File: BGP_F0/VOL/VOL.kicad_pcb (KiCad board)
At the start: 2 copper layers, 20 x 26 mm, 4 parts, among them J1 Conn_01x03_Female, J2 Conn_01x03_Female, P1 CONN_01X02

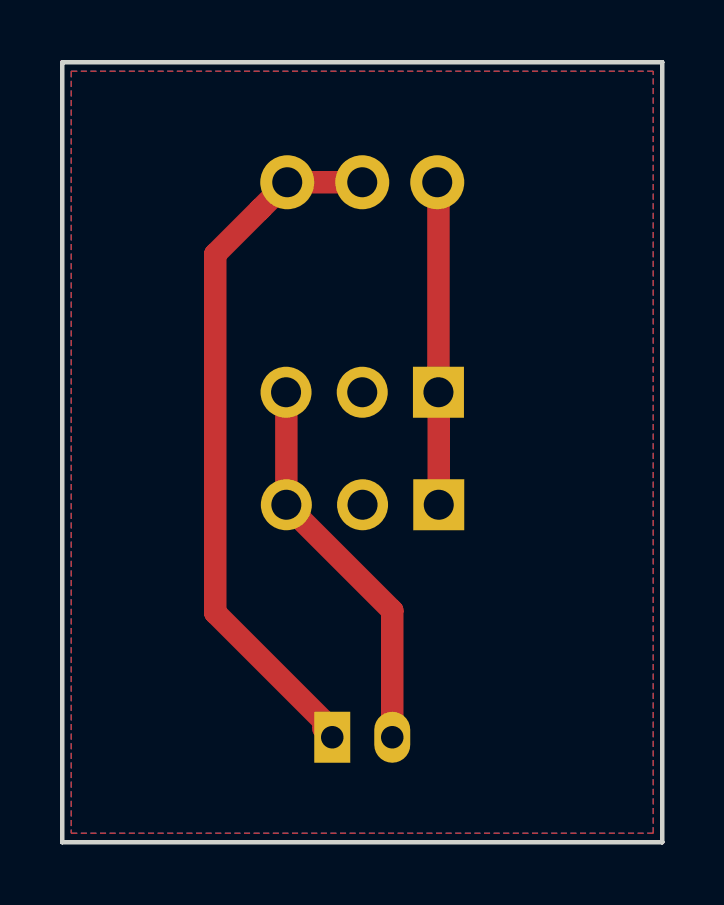
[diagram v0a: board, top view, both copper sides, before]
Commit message: Mid Buff
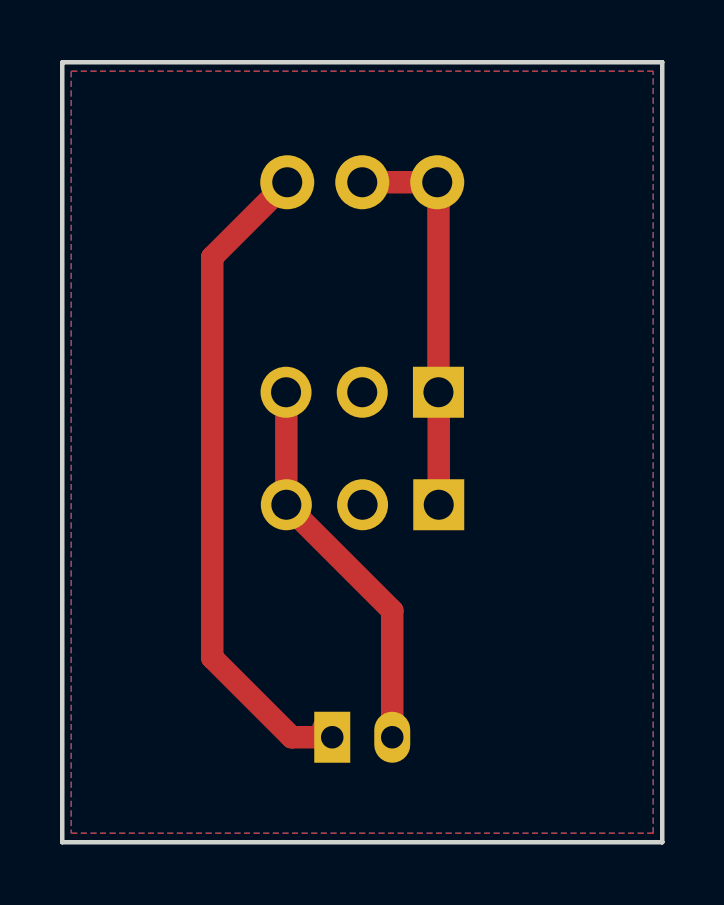
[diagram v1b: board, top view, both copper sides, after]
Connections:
- RV1 pad 2: /VOL_1 -> Net-(J1-Pad1)
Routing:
- net Net-(J1-Pad1): track 10.8 -> 13.3 mm
- net /VOL_1: track 24.0 -> 22.7 mm
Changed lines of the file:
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@@
   (general
     (links 6)
-    (no_connects 6)
+    (no_connects 0)
     (area 137.924999 75.924999 158.075001 102.075001)
     (thickness 1.6)
@@
       (net 3 "Net-(J1-Pad1)"))
     (pad 2 thru_hole circle (at 0 2.5 90) (size 1.8 1.8) (drill 1) (layers *.Cu *.Mask)
-      (net 1 /VOL_1))
+      (net 3 "Net-(J1-Pad1)"))
     (pad 1 thru_hole circle (at 0 0 90) (size 1.8 1.8) (drill 1) (layers *.Cu *.Mask)
       (net 1 /VOL_1))
@@
   (gr_line (start 138 76) (end 138 102) (layer Edge.Cuts) (width 0.15))
   (gr_line (start 158 76) (end 138 76) (layer Edge.Cuts) (width 0.15))
+  (segment (start 143 95.85) (end 143 82.5) (width 0.75) (layer F.Cu) (net 1))
+  (segment (start 143 82.5) (end 145.5 80) (width 0.75) (layer F.Cu) (net 1))
+  (segment (start 147 98.5) (end 145.65 98.5) (width 0.75) (layer F.Cu) (net 1))
+  (segment (start 145.65 98.5) (end 143 95.85) (width 0.75) (layer F.Cu) (net 1))
   (segment (start 147 98.5) (end 147 98.25) (width 0.75) (layer F.Cu) (net 1))
-  (segment (start 147 98.25) (end 143.1 94.35) (width 0.75) (layer F.Cu) (net 1))
-  (segment (start 143.1 94.35) (end 143.1 82.4) (width 0.75) (layer F.Cu) (net 1))
-  (segment (start 143.1 82.4) (end 144.600001 80.899999) (width 0.75) (layer F.Cu) (net 1))
-  (segment (start 144.600001 80.899999) (end 145.5 80) (width 0.75) (layer F.Cu) (net 1))
-  (segment (start 145.5 80) (end 148 80) (width 0.75) (layer F.Cu) (net 1))
   (segment (start 147 98.5) (end 146.7 98.2) (width 0.75) (layer F.Cu) (net 1))
   (segment (start 145.47 90.75) (end 145.47 87.01) (width 0.75) (layer F.Cu) (net 2))
@@
   (segment (start 149 98.5) (end 149 94.28) (width 0.75) (layer F.Cu) (net 2))
   (segment (start 149 94.28) (end 145.47 90.75) (width 0.75) (layer F.Cu) (net 2))
+  (segment (start 150.5 80) (end 148 80) (width 0.75) (layer F.Cu) (net 3))
   (segment (start 150.54 87) (end 150.54 80.04) (width 0.75) (layer F.Cu) (net 3))
   (segment (start 150.54 80.04) (end 150.5 80) (width 0.75) (layer F.Cu) (net 3))
